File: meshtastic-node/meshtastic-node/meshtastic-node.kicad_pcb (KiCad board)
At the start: 4 copper layers, 150.1 x 50 mm, 112 parts, among them IC1 CH224K, IC2 CN3791, IC3 SKY65313-21, IC4 TPS2121RUXT, IC5 Wio-WM1110, IC7 TPS2121RUXT, J1 USB_C_Receptacle_USB2.0, J2 Conn_01x05_Socket, J3 Conn_Coaxial_Small, J4 Conn_01x02_Socket, J5 Conn_01x02_Socket, J6 Conn_ARM_JTAG_SWD_10, Q1 PMOS, Q2 PMOS, SW2 SW_Push, SW3 SW_DPDT_x2, U1 TPS565208, U2 TPS61222DCK, U3 TPS61222DCK, U4 BME280, U5 INA3221, U6 USBLC6-2SC6

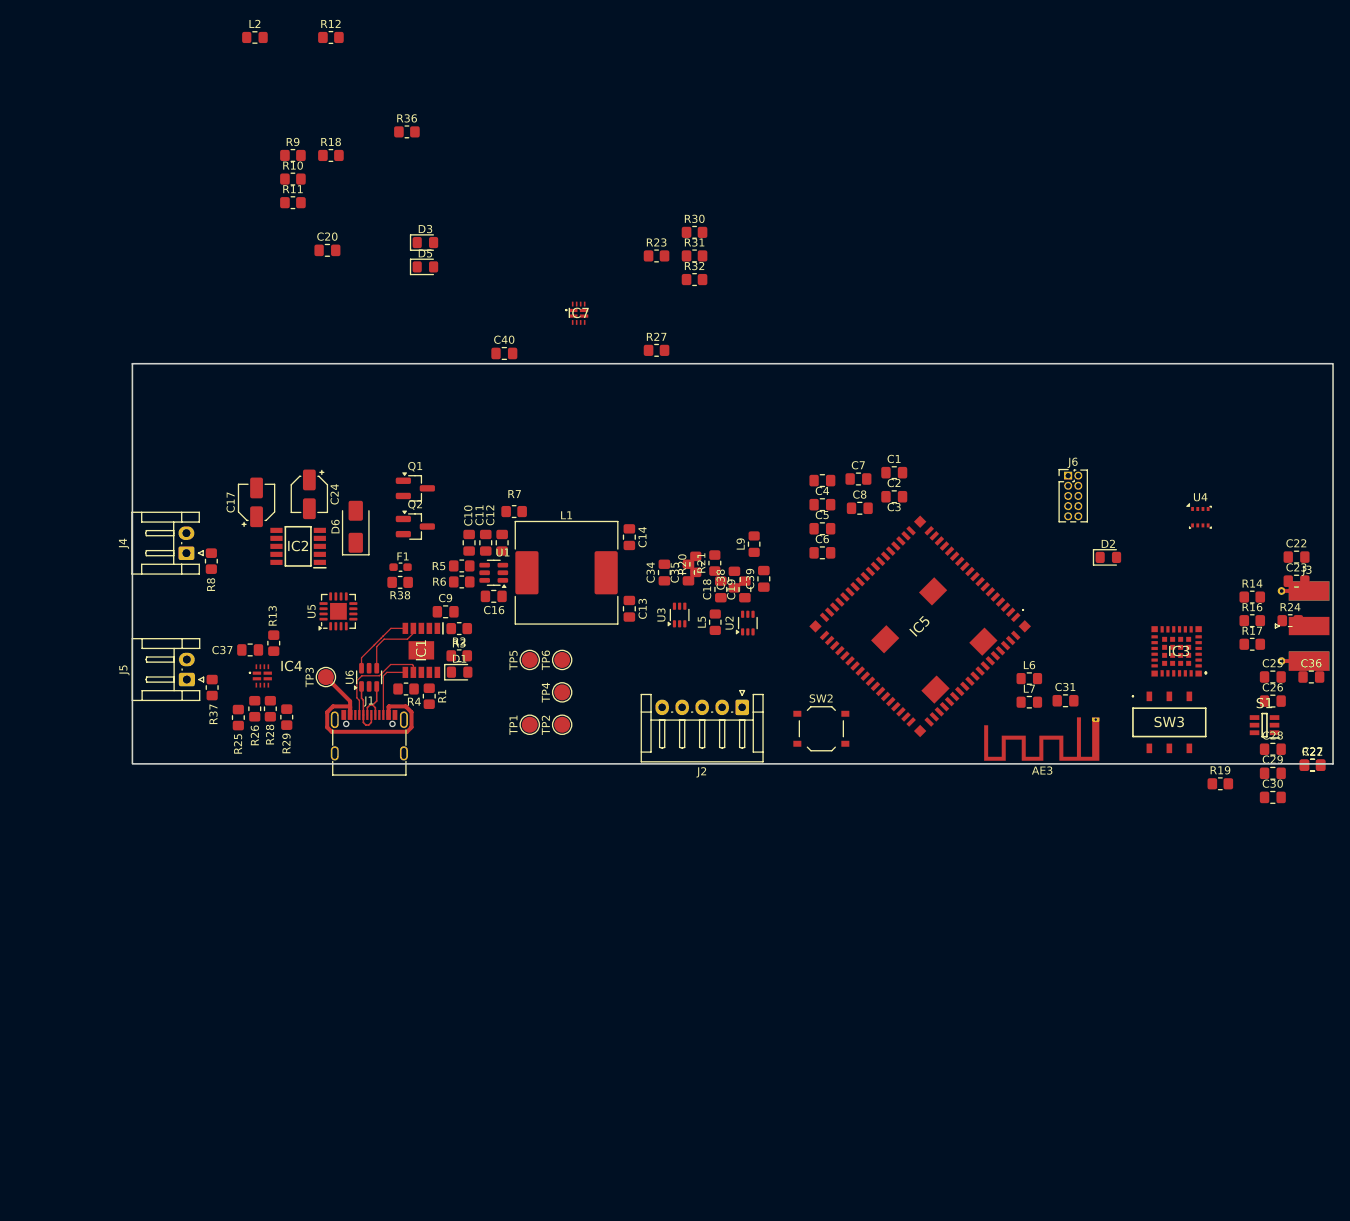
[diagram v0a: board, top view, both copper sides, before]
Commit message: routing
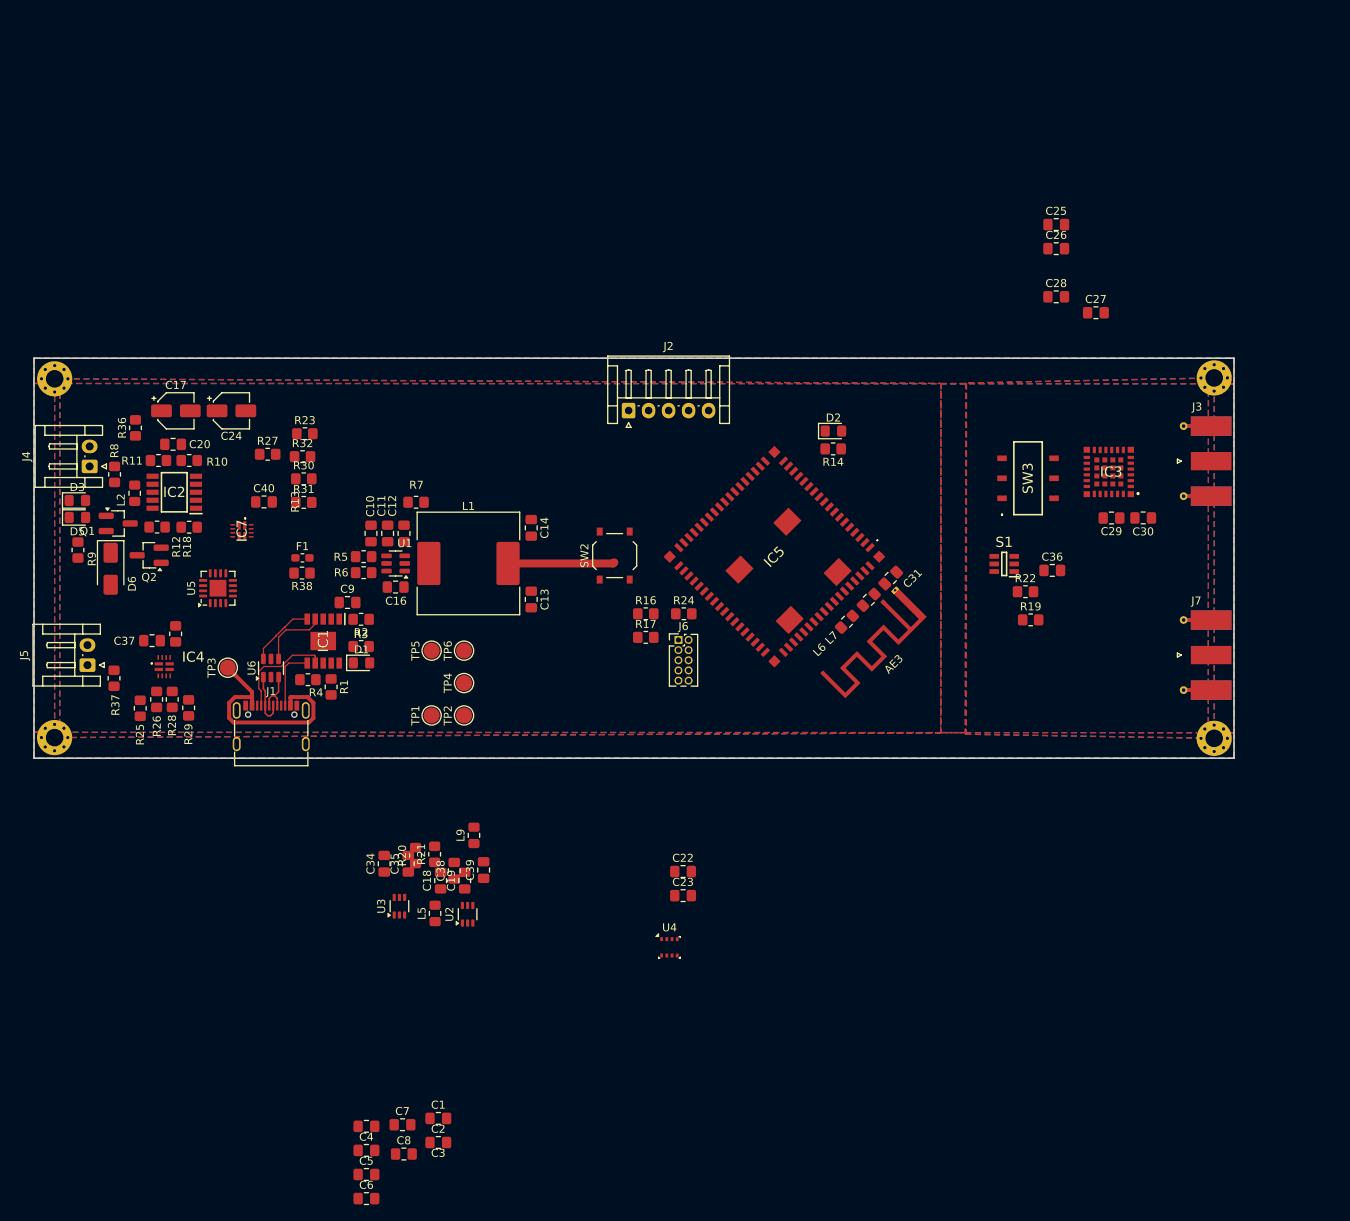
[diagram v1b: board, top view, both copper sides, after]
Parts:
- added J7: Conn_Coaxial_Small, Connector_Coaxial:SMA_Molex_73251-1153_EdgeMount_Horizontal, F.Cu at (178.6, 108.2)
- added REF**: MountingHole_2.2mm_M2_Pad_Via, MountingHole:MountingHole_2.2mm_M2_Pad_Via, F.Cu at (180.7, 118.6)
- added REF**: MountingHole_2.2mm_M2_Pad_Via, MountingHole:MountingHole_2.2mm_M2_Pad_Via, F.Cu at (35.8, 118.6)
- added REF**: MountingHole_2.2mm_M2_Pad_Via, MountingHole:MountingHole_2.2mm_M2_Pad_Via, F.Cu at (35.8, 73.7)
- added REF**: MountingHole_2.2mm_M2_Pad_Via, MountingHole:MountingHole_2.2mm_M2_Pad_Via, F.Cu at (180.7, 73.6)
- moved C1 98.8 mm to (83.7, 166.2)
- moved C2 98.8 mm to (83.7, 169.2)
- moved C5 98.8 mm to (74.7, 173.2)
- moved C6 98.8 mm to (74.7, 176.2)
- moved C7 98.8 mm to (79.2, 166.9)
- moved C8 98.8 mm to (79.4, 170.6)
- moved C3 98.8 mm to (74.7, 167.1)
- moved C4 98.8 mm to (74.7, 170.2)
- moved C22 86.2 mm to (114.3, 135.3)
- moved C23 86.2 mm to (114.3, 138.3)
- moved U4 85.4 mm to (112.6, 144.8)
- moved R16 75.8 mm to (109.7, 103.1)
- moved R17 75.8 mm to (109.7, 106.0)
- moved R24 75.8 mm to (114.4, 103.1)
- moved R12 64.9 mm to (48.6, 92.2), turned to 180 degrees
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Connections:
- C25 pad 1: +4V -> USE_ANT_2
- C26 pad 1: +4V -> USE_ANT_2
- C27 pad 1: +4V -> USE_ANT_2
- C28 pad 1: +4V -> USE_ANT_2
- IC3 pad 23: +4V -> USE_ANT_2
- IC3 pad 24: +4V -> USE_ANT_2
- IC3 pad 25: +4V -> USE_ANT_2
- IC3 pad 26: +4V -> USE_ANT_2
- SW3 pad 2: VDD_NRF -> +4V
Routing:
- net VDD_NRF: track 0.00 -> 13.3 mm
- added copper zone on B.Cu, net GND
- added copper zone on F.Cu, net GND
- added copper zone on In1.Cu, net GND
- added copper zone on In2.Cu, net GND
- added copper zone on In1.Cu, net VDD_NRF
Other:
- board size 150.1 x 50 mm -> 150 x 50 mm
